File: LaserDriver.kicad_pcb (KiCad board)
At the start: 2 copper layers, 40.2 x 40.5 mm, 31 parts, among them J100 Screw_Terminal_01x04, J101 Screw_Terminal_01x02, J102 nano_left, J103 nano_right, U100 TPS92513DGQR

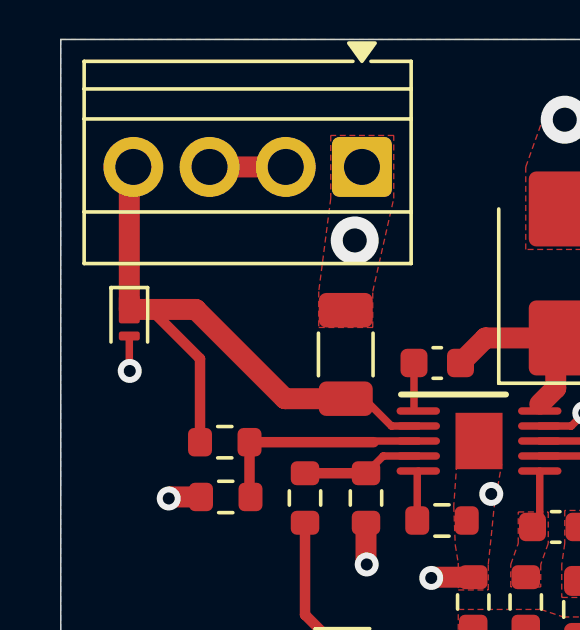
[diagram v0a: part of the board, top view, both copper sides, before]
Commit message: finished BOM
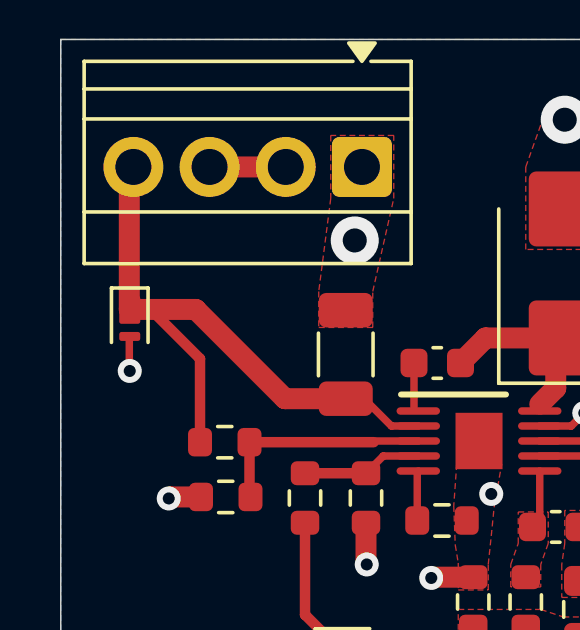
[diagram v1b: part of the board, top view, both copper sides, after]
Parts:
- D100: value PTVS12VZ1USK -> PTVS20VZ1USK
- D102, D103, D104: value PTVS5V0Z1USK -> PTVS10VZ1USK
- moved D103 11.4 mm to (50.4, 117.2)
- moved D104 11.4 mm to (39.0, 117.2)
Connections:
- D103 pad 1: /ard_PWM -> /ard_DAC
- D104 pad 1: /ard_DAC -> /ard_PWM
